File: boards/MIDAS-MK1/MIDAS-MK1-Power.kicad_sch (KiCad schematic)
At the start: 43 parts, among them U301 TPS2121, U302 TI_TPS566242DRLR, U303 TI_TPS566242DRLR

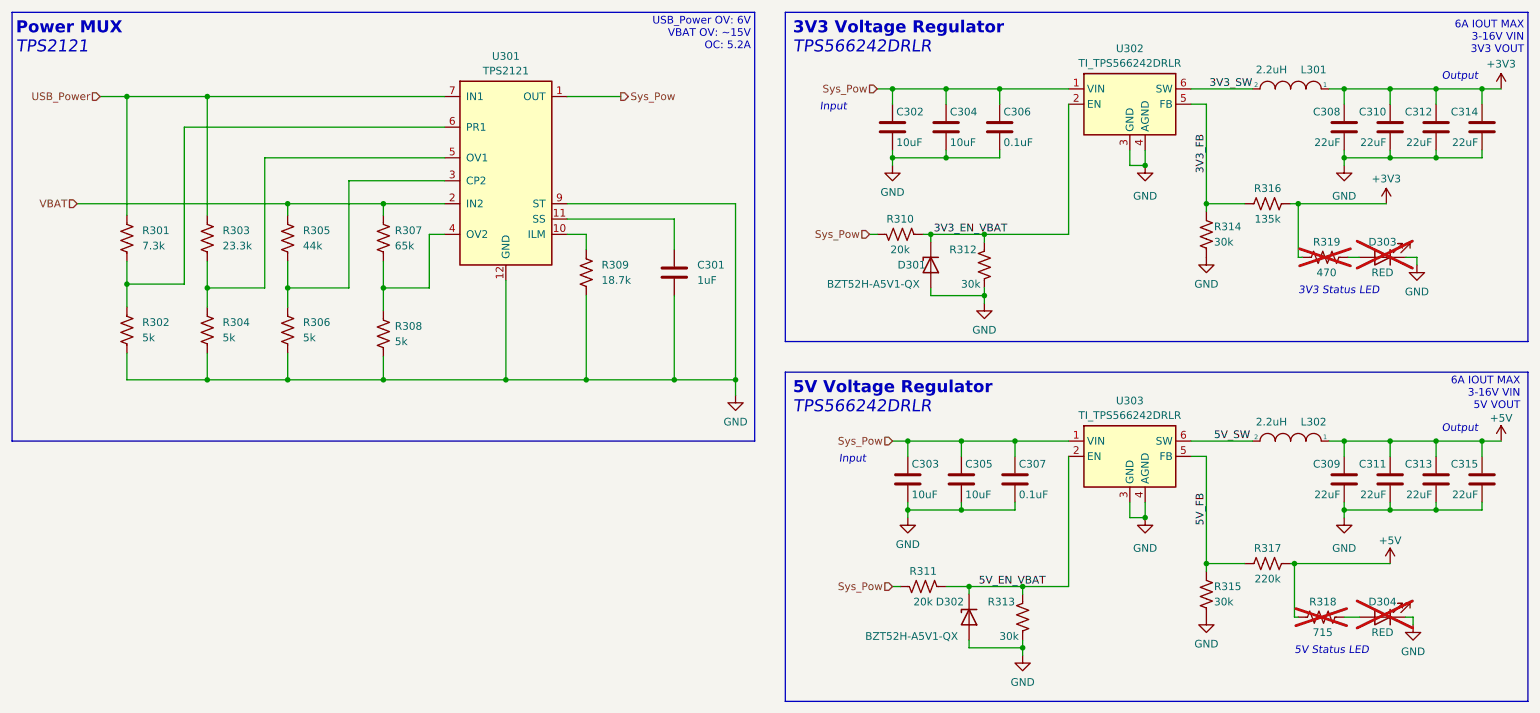
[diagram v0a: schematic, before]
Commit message: updated sch files for review
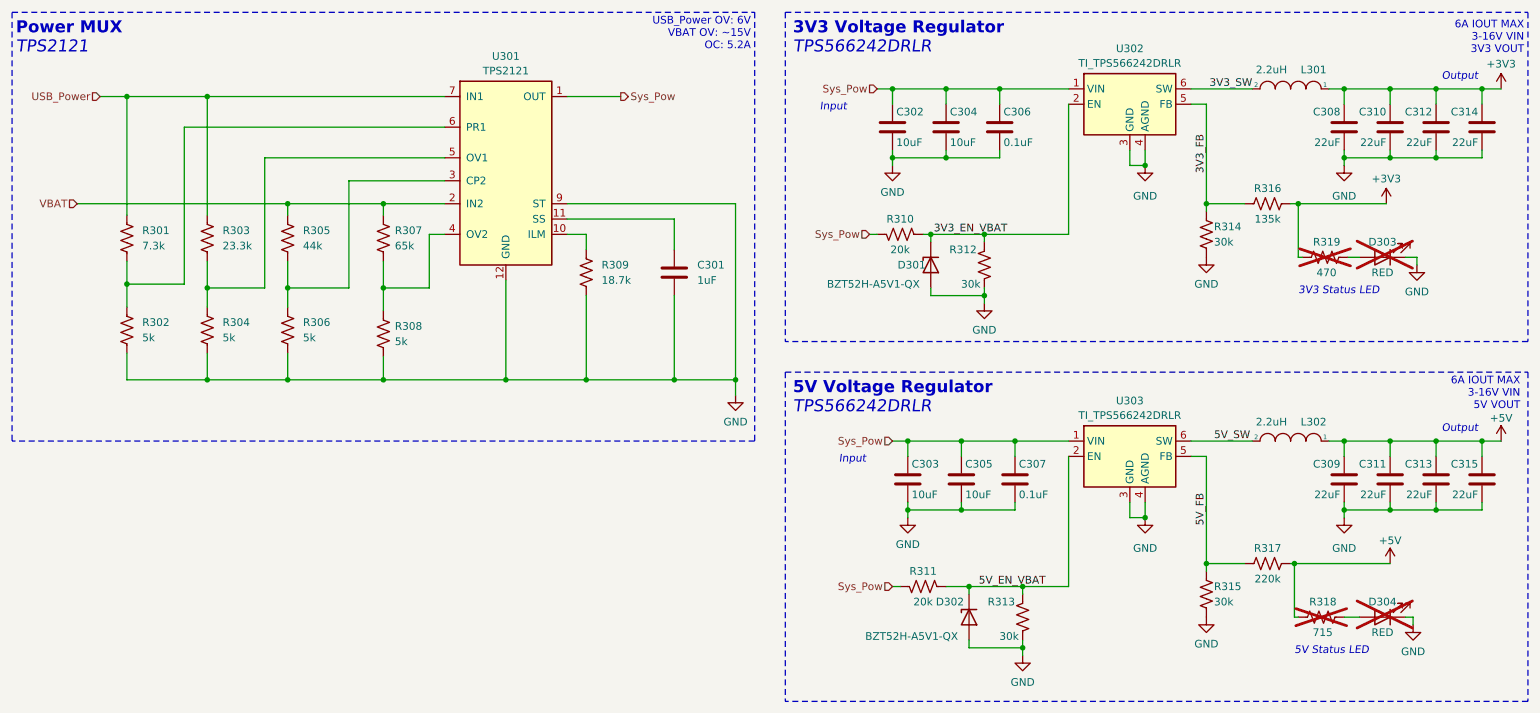
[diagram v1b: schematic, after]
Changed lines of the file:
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@@
   )
   (polyline (pts (xy 215.9 156.21) (xy 339.09 156.21))
-    (stroke (width 0) (type default))
+    (stroke (width 0) (type dash))
   )
   (wire (pts (xy 143.51 142.24) (xy 133.35 142.24))
@@
   )
   (polyline (pts (xy 339.09 156.21) (xy 339.09 210.82))
-    (stroke (width 0) (type default))
+    (stroke (width 0) (type dash))
   )
   (wire (pts (xy 273.05 177.8) (xy 273.05 180.34))
@@
   )
   (polyline (pts (xy 339.09 96.52) (xy 339.09 151.13))
-    (stroke (width 0) (type default))
+    (stroke (width 0) (type dash))
   )
   (wire (pts (xy 323.85 179.07) (xy 316.23 179.07))
@@
   )
   (polyline (pts (xy 87.63 96.52) (xy 87.63 167.64))
-    (stroke (width 0) (type default))
+    (stroke (width 0) (type dash))
   )
   (wire (pts (xy 233.68 120.65) (xy 242.57 120.65))
@@
   )
   (polyline (pts (xy 210.82 96.52) (xy 210.82 167.64))
-    (stroke (width 0) (type default))
+    (stroke (width 0) (type dash))
   )
   (wire (pts (xy 316.23 109.22) (xy 308.61 109.22))
@@
   )
   (polyline (pts (xy 210.82 167.64) (xy 87.63 167.64))
-    (stroke (width 0) (type default))
+    (stroke (width 0) (type dash))
   )
   (wire (pts (xy 233.68 120.65) (xy 233.68 121.92))
@@
   )
   (polyline (pts (xy 87.63 96.52) (xy 210.82 96.52))
-    (stroke (width 0) (type default))
+    (stroke (width 0) (type dash))
   )
   (wire (pts (xy 308.61 121.92) (xy 308.61 120.65))
@@
   )
   (polyline (pts (xy 339.09 151.13) (xy 215.9 151.13))
-    (stroke (width 0) (type default))
+    (stroke (width 0) (type dash))
   )
   (wire (pts (xy 116.205 115.57) (xy 159.385 115.57))
@@
   )
   (polyline (pts (xy 215.9 96.52) (xy 215.9 151.13))
-    (stroke (width 0) (type default))
+    (stroke (width 0) (type dash))
   )
   (wire (pts (xy 308.61 196.85) (xy 311.15 196.85))
@@
   )
   (polyline (pts (xy 215.9 156.21) (xy 215.9 210.82))
-    (stroke (width 0) (type default))
+    (stroke (width 0) (type dash))
   )
   (wire (pts (xy 316.23 167.64) (xy 308.61 167.64))
@@
   )
   (polyline (pts (xy 339.09 210.82) (xy 215.9 210.82))
-    (stroke (width 0) (type default))
+    (stroke (width 0) (type dash))
   )
   (wire (pts (xy 309.245 137.16) (xy 311.15 137.16))
@@
   )
   (polyline (pts (xy 215.9 96.52) (xy 339.09 96.52))
-    (stroke (width 0) (type default))
+    (stroke (width 0) (type dash))
   )
   (wire (pts (xy 248.92 143.51) (xy 248.92 144.78))
